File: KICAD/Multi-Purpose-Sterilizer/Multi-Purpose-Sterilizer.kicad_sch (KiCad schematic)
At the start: 1 part, among them Q1 Q_NMOS_SGD

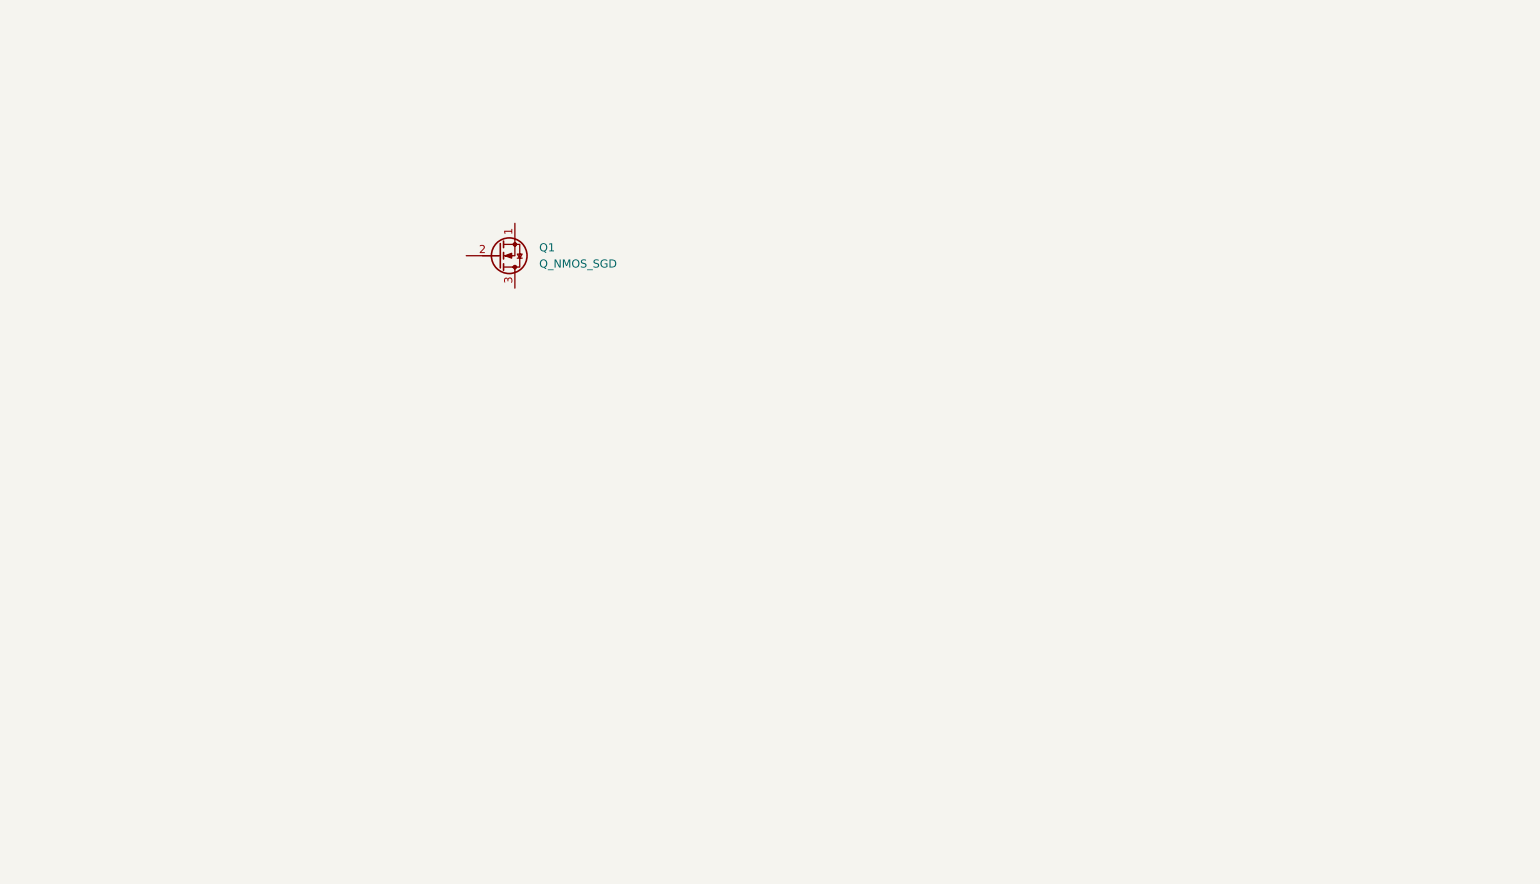
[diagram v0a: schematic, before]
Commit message: Update : KICAD - Schematic File
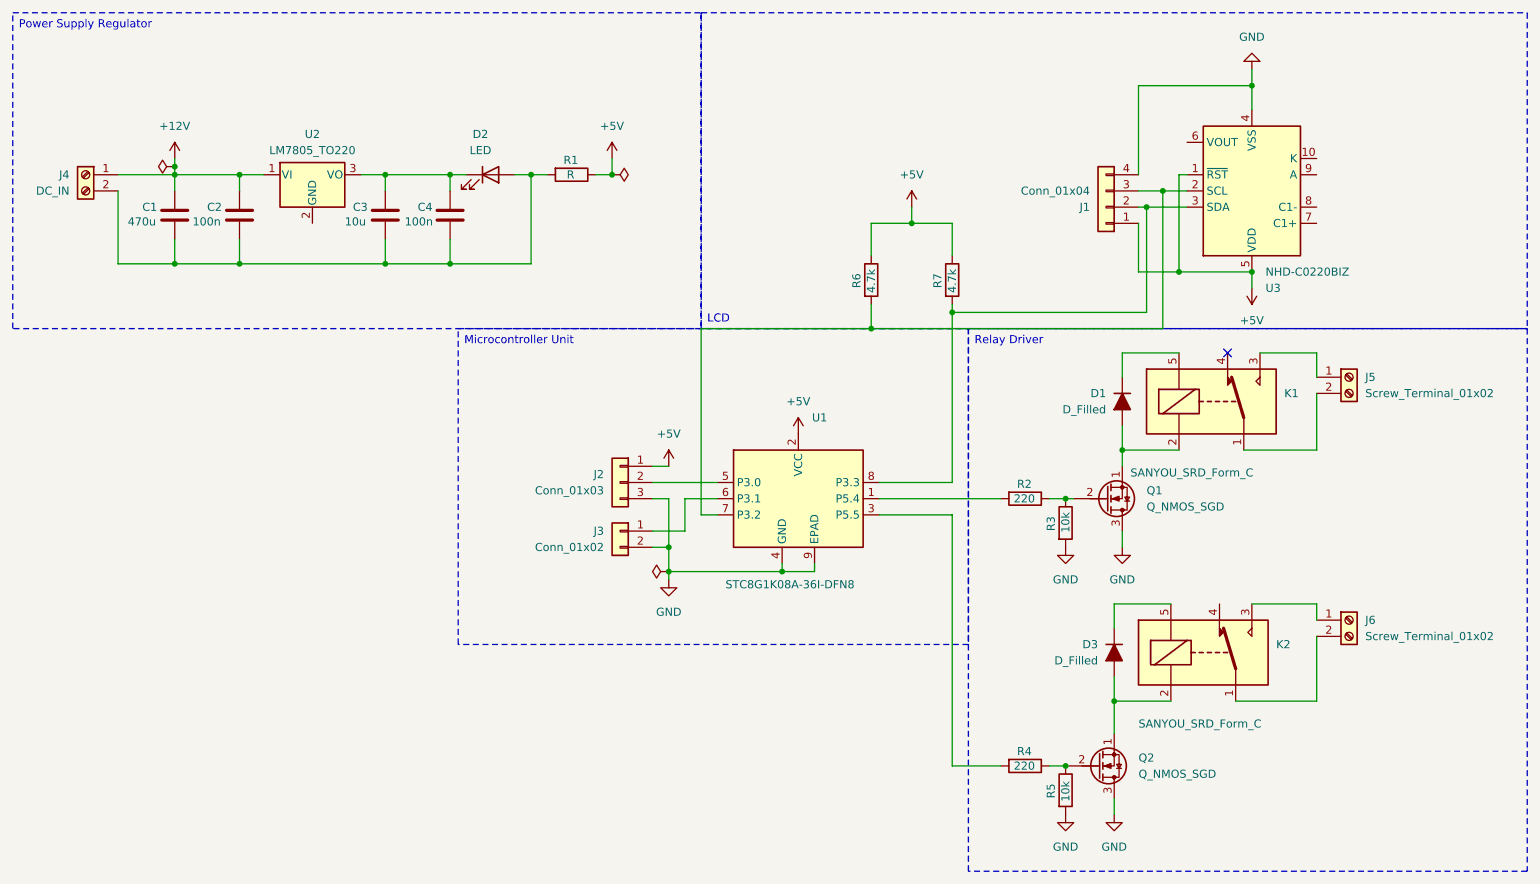
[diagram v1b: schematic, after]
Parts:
- added C1: 470u, symbol Device:C
- added C2, C4: 100n, symbol Device:C
- added C3: 10u, symbol Device:C
- added D1, D3: D_Filled, symbol Device:D_Filled
- added D2: LED, symbol Device:LED
- added J1: Conn_01x04, symbol Connector_Generic:Conn_01x04
- added J2: Conn_01x03, symbol Connector_Generic:Conn_01x03
- added J3: Conn_01x02, symbol Connector_Generic:Conn_01x02
- added J4: DC_IN, symbol Connector:Screw_Terminal_01x02
- added J5, J6: Screw_Terminal_01x02, symbol Connector:Screw_Terminal_01x02
- added K1, K2: SANYOU_SRD_Form_C, Relay_THT:Relay_SPDT_SANYOU_SRD_Series_Form_C, symbol Relay:SANYOU_SRD_Form_C
- added Q2: Q_NMOS_SGD, symbol Transistor_FET:Q_NMOS_SGD
- added R1: R, symbol Device:R
- added R2, R4: 220, symbol Device:R
- added R3, R5: 10k, symbol Device:R
- added R6, R7: 4.7k, symbol Device:R
- added U1: STC8G1K08A-36I-DFN8, Package_DFN_QFN:DFN-8-1EP_3x3mm_P0.5mm_EP1.7x2.4mm, symbol MCU_STC:STC8G1K08A-36I-DFN8
- added U2: LM7805_TO220, Package_TO_SOT_THT:TO-220-3_Vertical, symbol Regulator_Linear:LM7805_TO220
- added U3: NHD-C0220BIZ, Display:NHD-C0220BiZ, symbol Display_Character:NHD-C0220BIZ
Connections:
- net at Q1.1 (S): now also D1.2 (A), K1.2
- net at Q1.2 (G): now also R2.1, R3.1
- net GND: now reaches Q1.3 (D)
- net GND: now also J1.4 (Pin_4), J2.3 (Pin_3), J3.2 (Pin_2), Q2.3 (D), R3.2, R5.2, U1.4 (GND), U1.9 (EPAD), U3.4 (VSS)
- new net: J1.2 (Pin_2), R7.2, U1.8 (P3.3), U3.3 (SDA)
- new net: D3.1 (K), K2.5
- new net: D3.2 (A), K2.2, Q2.1 (S)
- new net: J1.3 (Pin_3), R6.2, U1.7 (P3.2), U3.2 (SCL)
- new net: Q2.2 (G), R4.1, R5.1
- new net: C3.1, C4.1, D2.1 (K), U2.3 (VO)
- new net: J3.1 (Pin_1), U1.6 (P3.1)
- new net: C1.2, C2.2, C3.2, C4.2, D2.2 (A), J4.2 (Pin_2), R1.2
- new net: J2.2 (Pin_2), U1.5 (P3.0)
- new net: R2.2, U1.1 (P5.4)
- new net: J5.2 (Pin_2), K1.1
- new net: J5.1 (Pin_1), K1.3
- new net: D1.1 (K), K1.5
- new net: R4.2, U1.3 (P5.5)
- new net: J6.1 (Pin_1), K2.3
- new net: J6.2 (Pin_2), K2.1
- new net +12V: C1.1, C2.1, J4.1 (Pin_1), U2.1 (VI)
- new net +5V: J1.1 (Pin_1), J2.1 (Pin_1), R1.1, R6.1, R7.1, U1.2 (VCC), U3.1 (~{RST}), U3.5 (VDD)
- no-connect marks 0 -> 1
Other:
- moved on the sheet: Q1
